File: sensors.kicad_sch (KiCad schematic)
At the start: 5 parts, among them U3 ICM-42688-P, U4 NEO-M8M

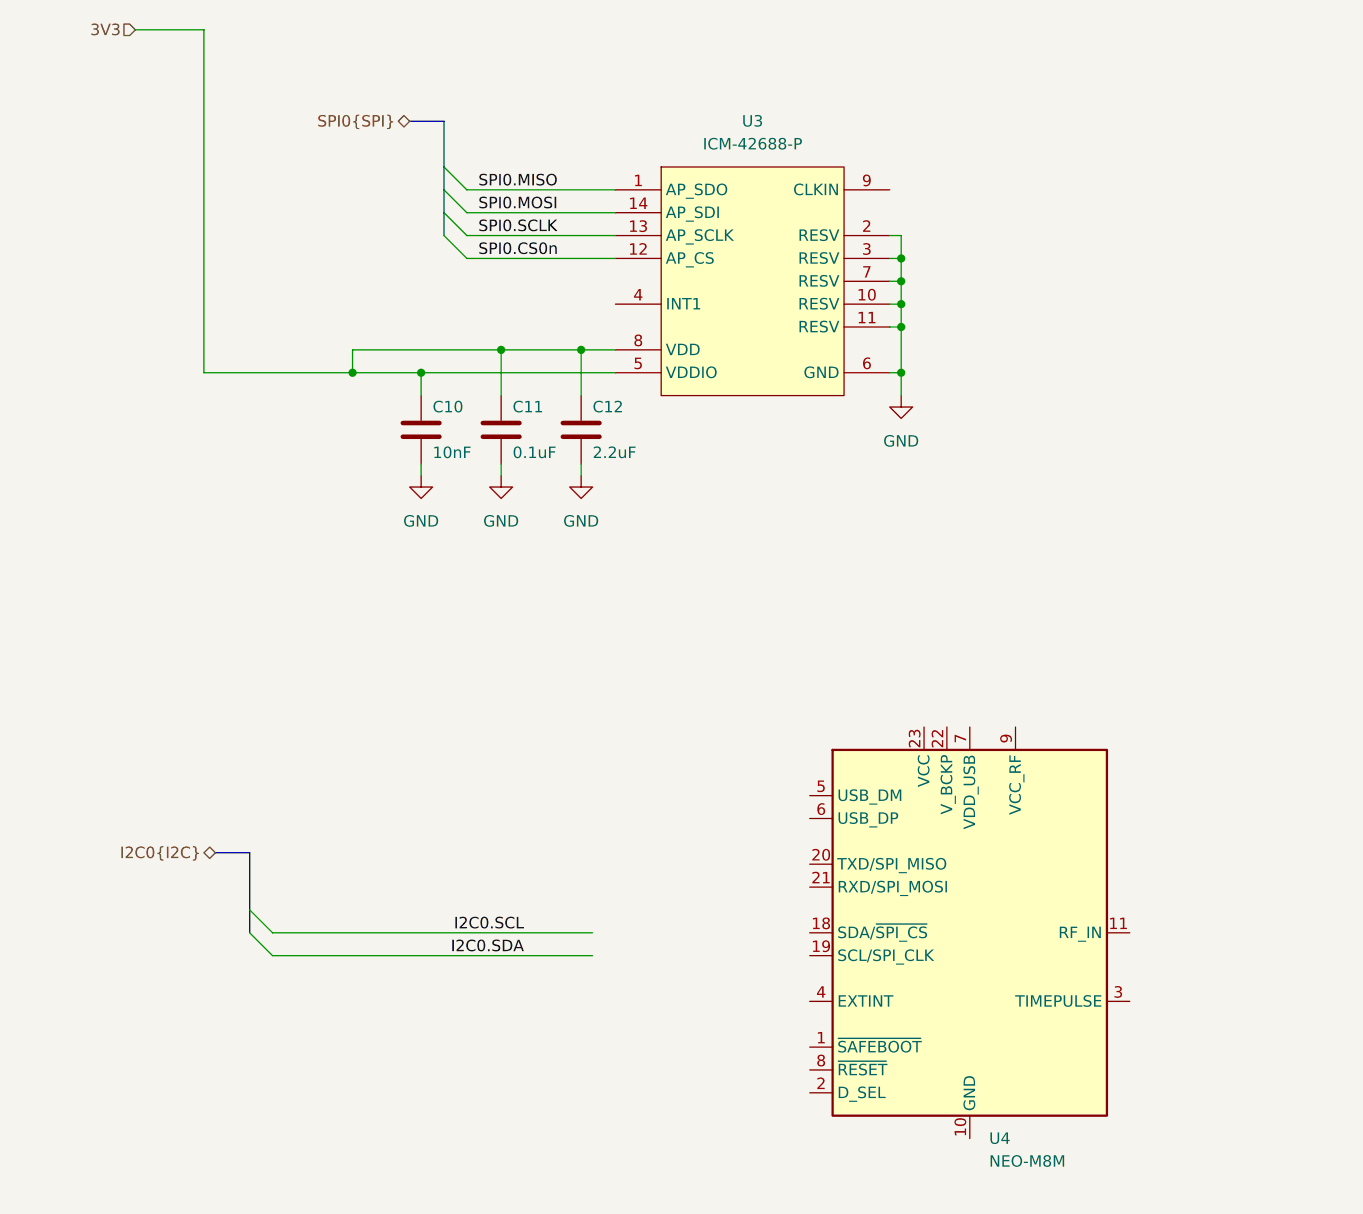
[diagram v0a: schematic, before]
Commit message: neo m8m impl.
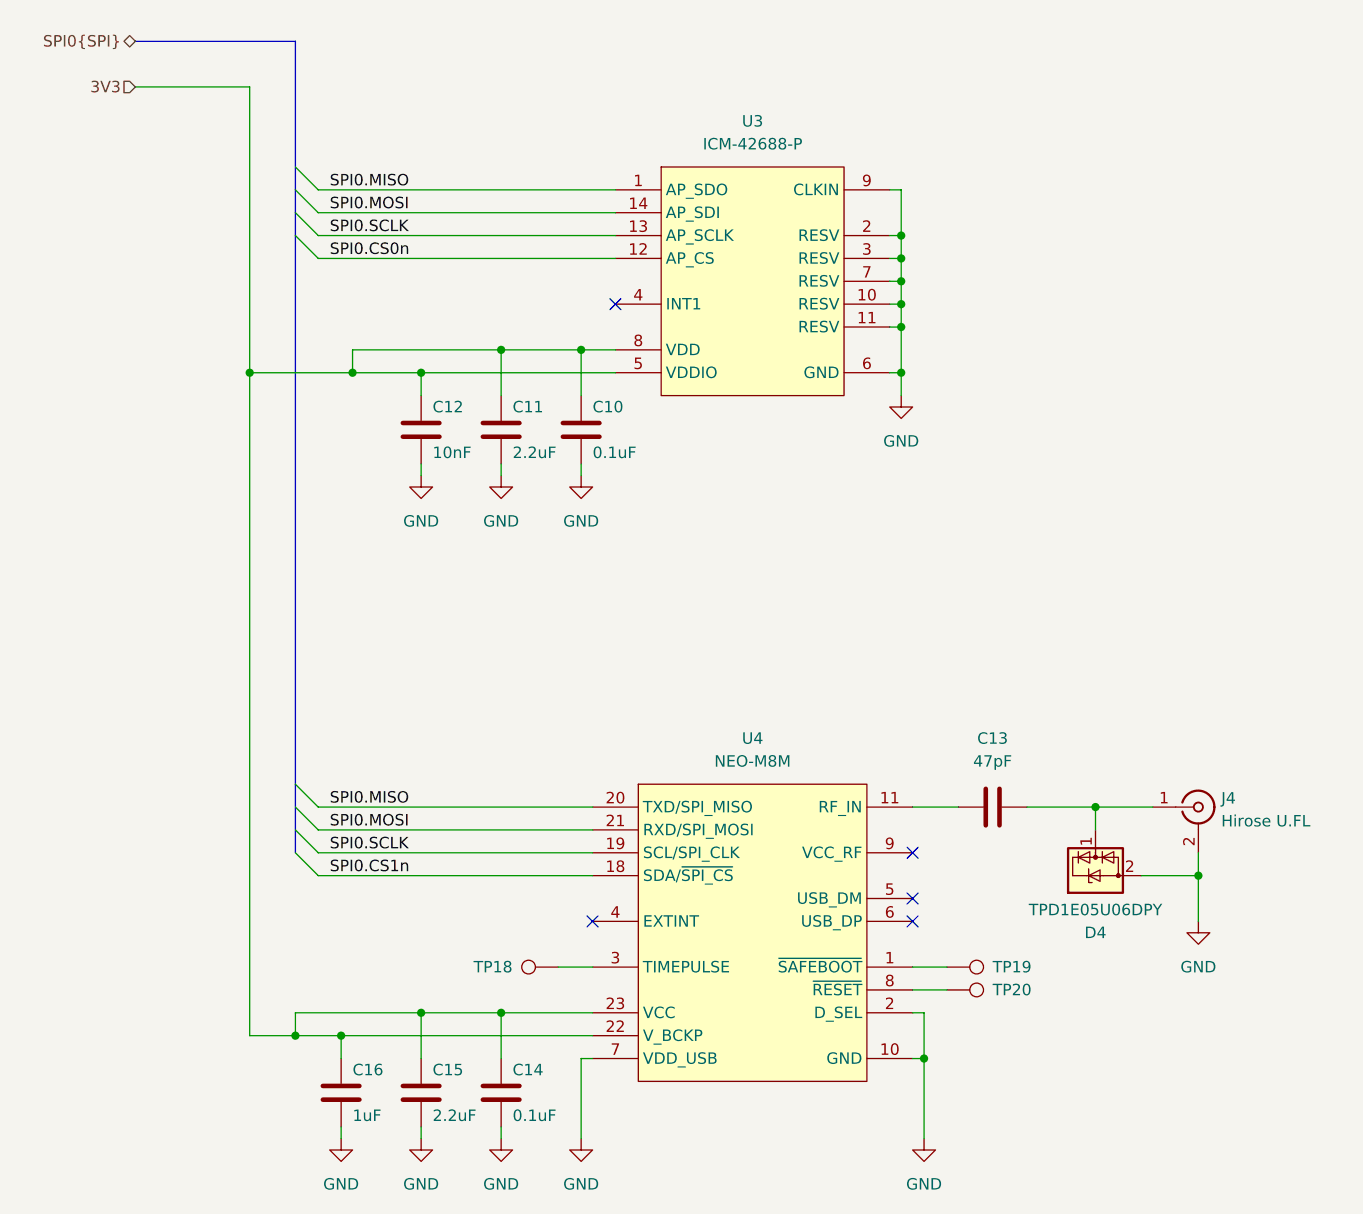
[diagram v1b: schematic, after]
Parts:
- added C13: 47pF, symbol Device:C
- added C14: 0.1uF, Capacitor_SMD:C_0402_1005Metric, symbol library:C
- added C15: 2.2uF, Capacitor_SMD:C_0402_1005Metric, symbol library:C
- added C16: 1uF, Capacitor_SMD:C_0402_1005Metric, symbol library:C
- added D4: TPD1E05U06DPY, Package_SON:Texas_DPY0002A_0.6x1mm_P0.65mm, symbol Power_Protection:TPD1E05U06DPY
- added J4: Hirose U.FL, Connector_Coaxial:U.FL_Hirose_U.FL-R-SMT-1_Vertical, symbol Connector:Conn_Coaxial
- added TP18, TP19, TP20: TestPoint, TestPoint:TestPoint_Pad_D1.0mm, symbol Connector:TestPoint
- renumbered C11 to C10, C12 to C11, C10 to C12
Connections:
- net 3V3: now also U4.22 (V_BCKP), U4.23 (VCC), C14.1, C15.1, C16.1
- net GND: now also U3.9 (CLKIN), U4.10 (GND), U4.14 (RESERVED), U4.2 (D_SEL), U4.7 (VDD_USB), C14.2, C15.2, C16.2, D4.2 (GND), J4.2 (Ext)
- net SPI0.MISO: now also U4.20 (TXD/SPI_MISO)
- net SPI0.MOSI: now also U4.21 (RXD/SPI_MOSI)
- net SPI0.SCLK: now also U4.19 (SCL/SPI_CLK)
- net at U4.1 (~{SAFEBOOT}): now also TP19.1
- net at U4.12 (GND), U4.13 (GND), U4.24 (GND): no longer U4.10 (GND)
- net at U4.11 (RF_IN): now also C13.1
- net at U4.15 (RESERVED): now also U4.16 (RESERVED), U4.17 (RESERVED)
- net SPI0.CS1n: now reaches U4.18 (SDA/~{SPI_CS})
- net at U4.3 (TIMEPULSE): now also TP18.1
- net at U4.8 (~{RESET}): now also TP20.1
- new net: C13.2, D4.1 (I/O), J4.1 (In)
- no-connect marks 0 -> 5
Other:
- moved on the sheet: C10, C11, U4
